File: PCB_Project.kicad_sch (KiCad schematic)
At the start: 0 parts

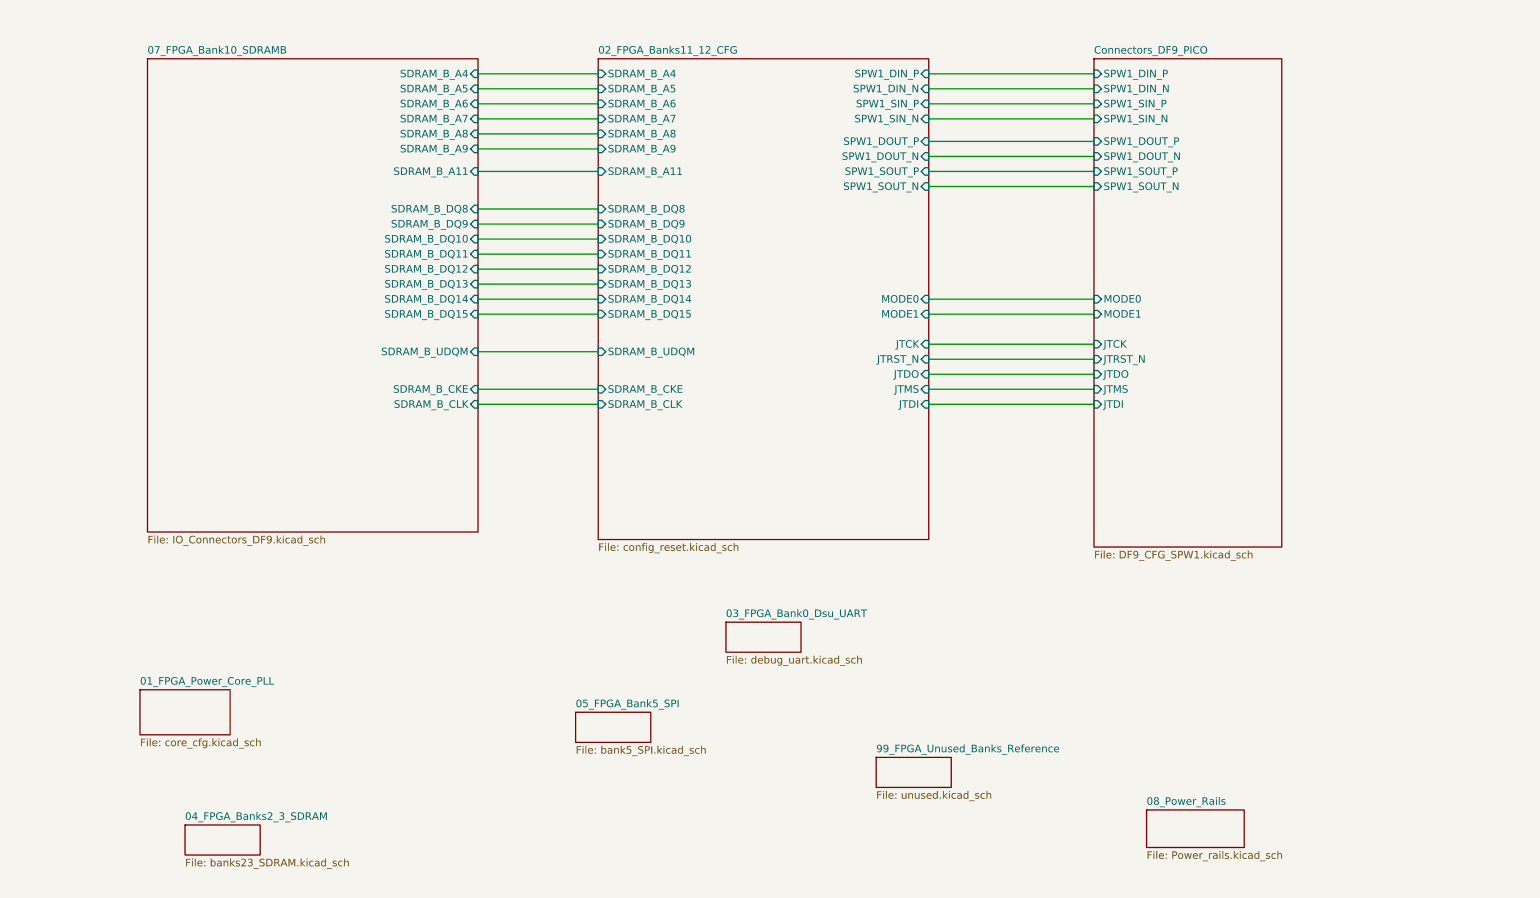
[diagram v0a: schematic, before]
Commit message: power tree
power tree defined. Few changes remaining but almost finalized
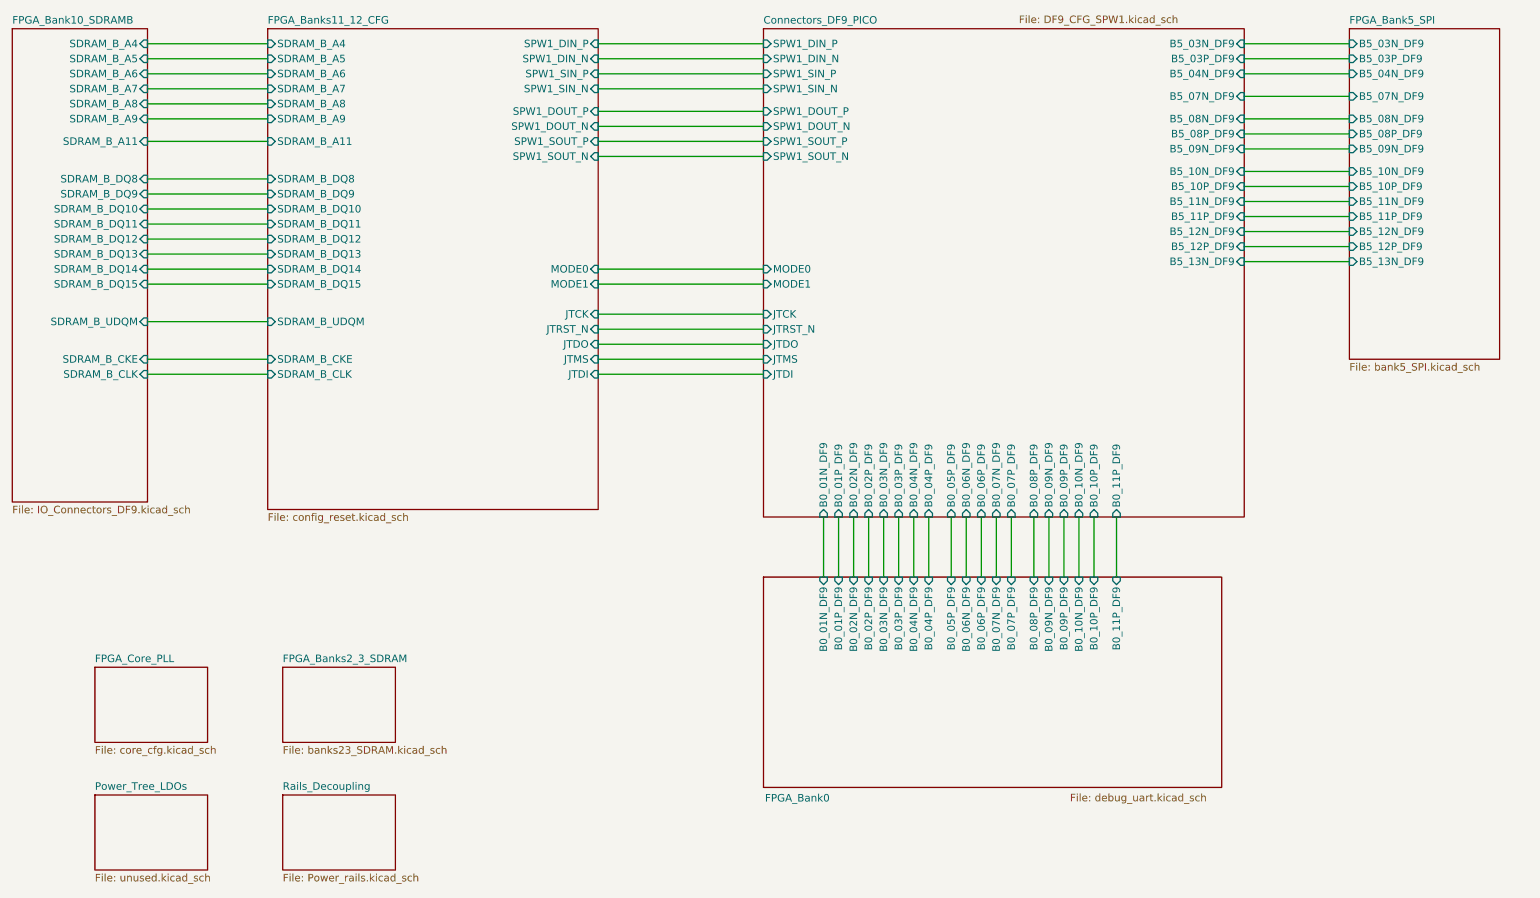
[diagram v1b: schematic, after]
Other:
- sheet 01_FPGA_Power_Core_PLL renamed FPGA_Core_PLL
- sheet 02_FPGA_Banks11_12_CFG renamed FPGA_Banks11_12_CFG
- sheet 03_FPGA_Bank0_Dsu_UART renamed FPGA_Bank0
- sheet 04_FPGA_Banks2_3_SDRAM renamed FPGA_Banks2_3_SDRAM
- sheet 05_FPGA_Bank5_SPI renamed FPGA_Bank5_SPI
- sheet 07_FPGA_Bank10_SDRAMB renamed FPGA_Bank10_SDRAMB
- sheet 08_Power_Rails renamed Rails_Decoupling
- sheet 99_FPGA_Unused_Banks_Reference renamed Power_Tree_LDOs
- sheet Connectors_DF9_PICO ports: added B0_01N_DF9, B0_01P_DF9, B0_02N_DF9, B0_02P_DF9, B0_03N_DF9, B0_03P_DF9, B0_04N_DF9, B0_04P_DF9, B0_05P_DF9, B0_06N_DF9, B0_06P_DF9, B0_07N_DF9, B0_07P_DF9, B0_08P_DF9, B0_09N_DF9, B0_09P_DF9, B0_10N_DF9, B0_10P_DF9, B0_11P_DF9, B5_03N_DF9, B5_03P_DF9, B5_04N_DF9, B5_07N_DF9, B5_08N_DF9, B5_08P_DF9, B5_09N_DF9, B5_10N_DF9, B5_10P_DF9, B5_11N_DF9, B5_11P_DF9, B5_12N_DF9, B5_12P_DF9, B5_13N_DF9; removed none
- sheet FPGA_Bank0 ports: added B0_01N_DF9, B0_01P_DF9, B0_02N_DF9, B0_02P_DF9, B0_03N_DF9, B0_03P_DF9, B0_04N_DF9, B0_04P_DF9, B0_05P_DF9, B0_06N_DF9, B0_06P_DF9, B0_07N_DF9, B0_07P_DF9, B0_08P_DF9, B0_09N_DF9, B0_09P_DF9, B0_10N_DF9, B0_10P_DF9, B0_11P_DF9; removed none
- sheet FPGA_Bank5_SPI ports: added B5_03N_DF9, B5_03P_DF9, B5_04N_DF9, B5_07N_DF9, B5_08N_DF9, B5_08P_DF9, B5_09N_DF9, B5_10N_DF9, B5_10P_DF9, B5_11N_DF9, B5_11P_DF9, B5_12N_DF9, B5_12P_DF9, B5_13N_DF9; removed none
